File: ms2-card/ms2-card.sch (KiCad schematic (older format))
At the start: 30 parts, among them J10 MicroSD_SPI_CD, J11 I2C, J20 Smartcard Connector, J21 Card Edge, J22 Card Edge, J23 Conn_01x04, J30 Power_Only, M1 PI_PICO_ZERO, Q30 BC847, SW1 SW_Push, U1 W25Q128JVS

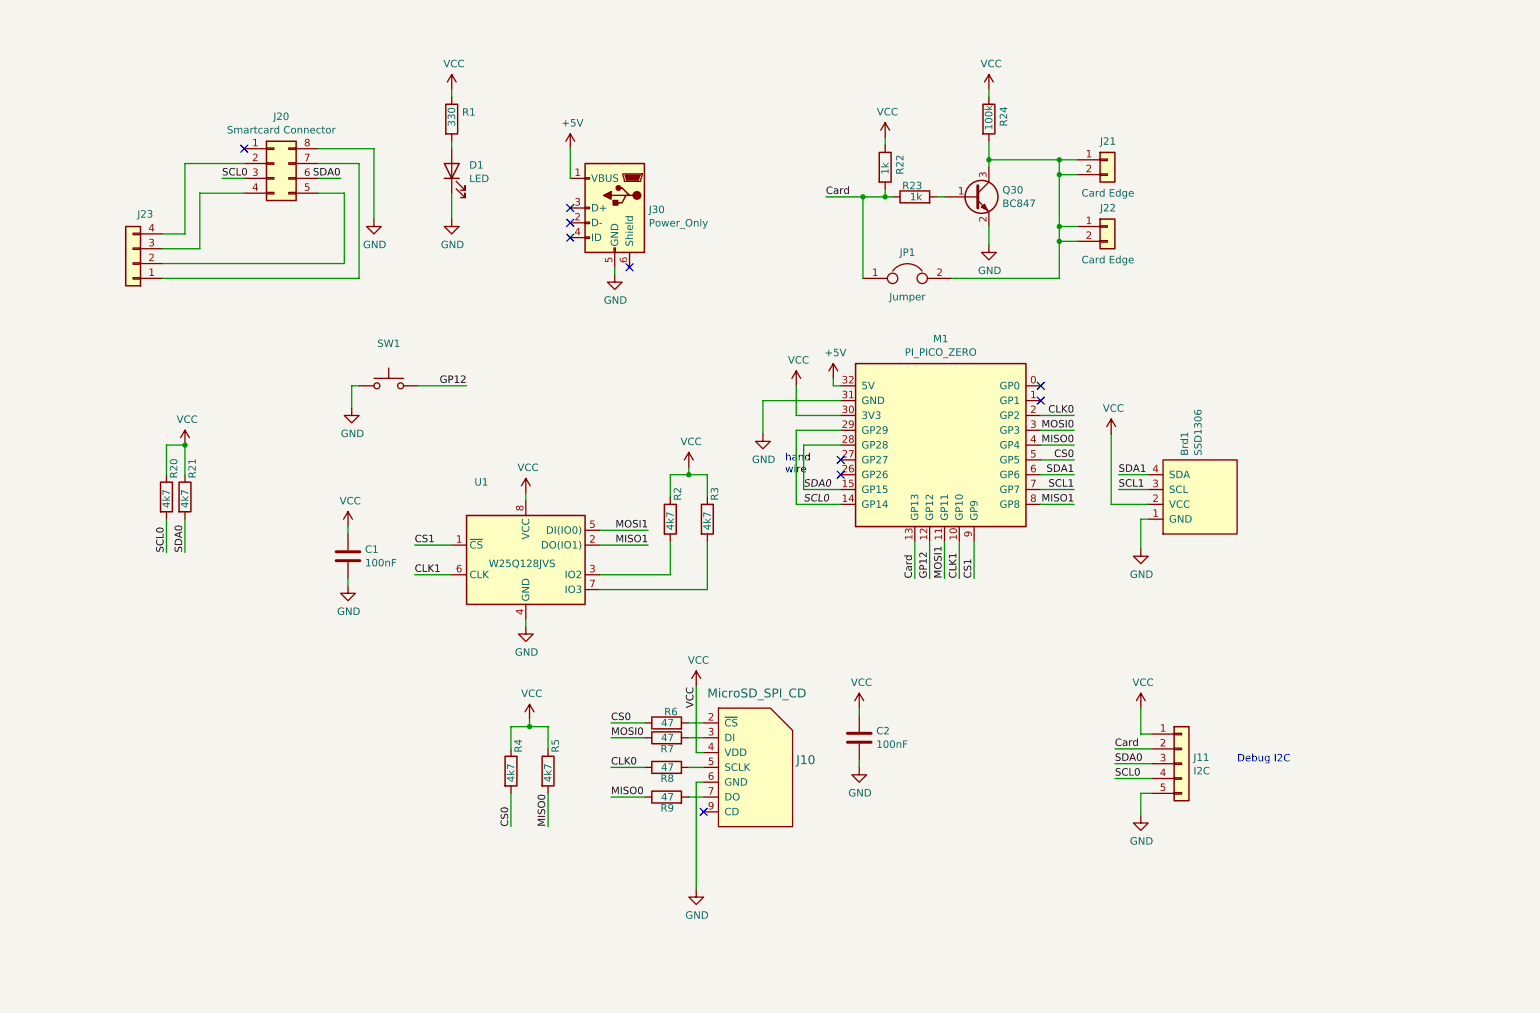
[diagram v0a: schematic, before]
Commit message: try to solve conflict
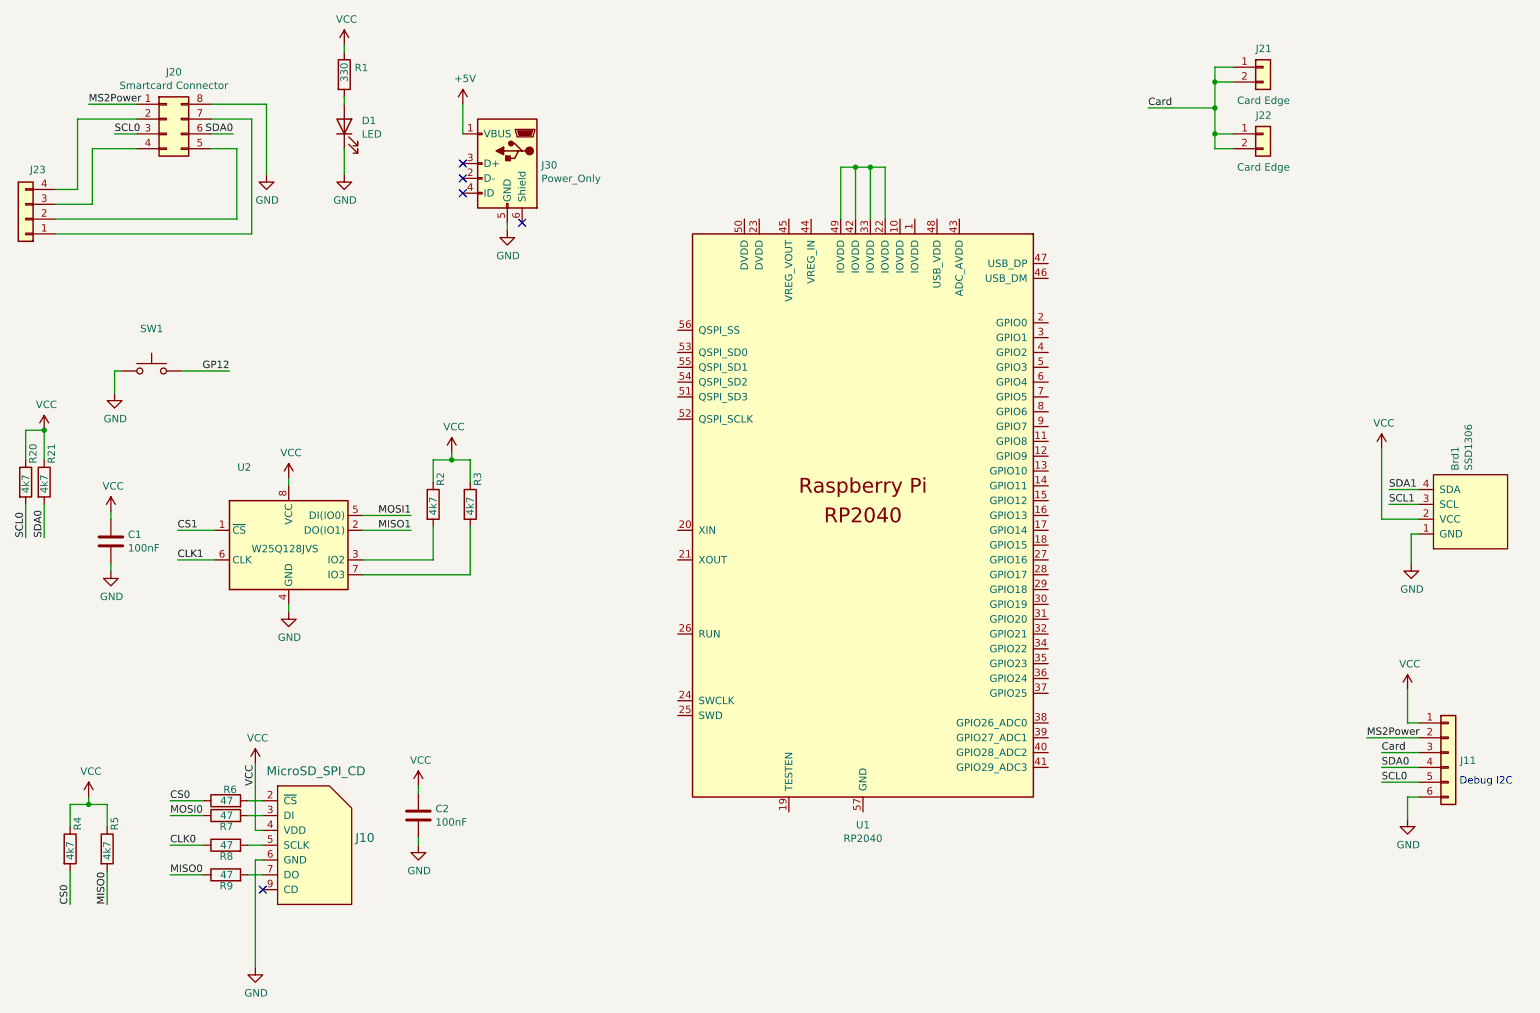
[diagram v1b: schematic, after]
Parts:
- removed J11: I2C, Connector_PinHeader_2.54mm:PinHeader_1x05_P2.54mm_Vertical, symbol Connector_Generic:Conn_01x05
- removed JP1: Jumper, Jumper:SolderJumper-2_P1.3mm_Open_TrianglePad1.0x1.5mm, symbol Device:Jumper
- removed M1: PI_PICO_ZERO, Lokkarten:PI_PICO_ZERO, symbol Lokkarten:PI_PICO_ZERO
- removed Q30: BC847, Package_TO_SOT_SMD:SOT-23, symbol Transistor_BJT:BC847
- removed R22, R23: 1k, Resistors_SMD:R_0805_HandSolderingII, symbol Device:R
- removed R24: 100k, Resistors_SMD:R_0805_HandSolderingII, symbol Device:R
- added J11: Conn_01x06, Connector_PinHeader_2.54mm:PinHeader_1x06_P2.54mm_Vertical, symbol Connector_Generic:Conn_01x06
- added U1: RP2040, RP2040:RP2040-QFN-56, symbol MCU_RaspberryPi_RP2040:RP2040
- R6, R7: footprint Resistors_SMD:R_0805_HandSolderingII -> Resistor_SMD:R_0603_1608Metric_Pad0.98x0.95mm_HandSolder
- U2: renamed from U1; JLCPCB (none) -> C97521
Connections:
- net Card: now also J21.1 (Pin_1), J21.2 (Pin_2), J22.1 (Pin_1), J22.2 (Pin_2), J11.3 (Pin_3)
- net GND: now also J11.6 (Pin_6)
- net SCL0: now also J11.5 (Pin_5)
- net SDA0: now also J11.4 (Pin_4)
- net VCC: now also J11.1 (Pin_1)
- net MS2Power: now reaches J20.1 (Pin_1)
- net MS2Power: now also J11.2 (Pin_2)
- new net: U1.22 (IOVDD), U1.33 (IOVDD), U1.42 (IOVDD), U1.49 (IOVDD)
- no-connect marks 10 -> 5
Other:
- note removed: "hand\nwire"
- moved on the sheet: Brd1, C1, C2, D1, J10, J20, J21, J22, J23, J30, R1, R2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
